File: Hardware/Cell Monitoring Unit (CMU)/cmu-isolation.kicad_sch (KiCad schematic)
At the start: 26 parts, among them T1 CEP99-102, T2 CEP99-102, U1 PESD5V0L2BT, U2 PESD5V0L2BT

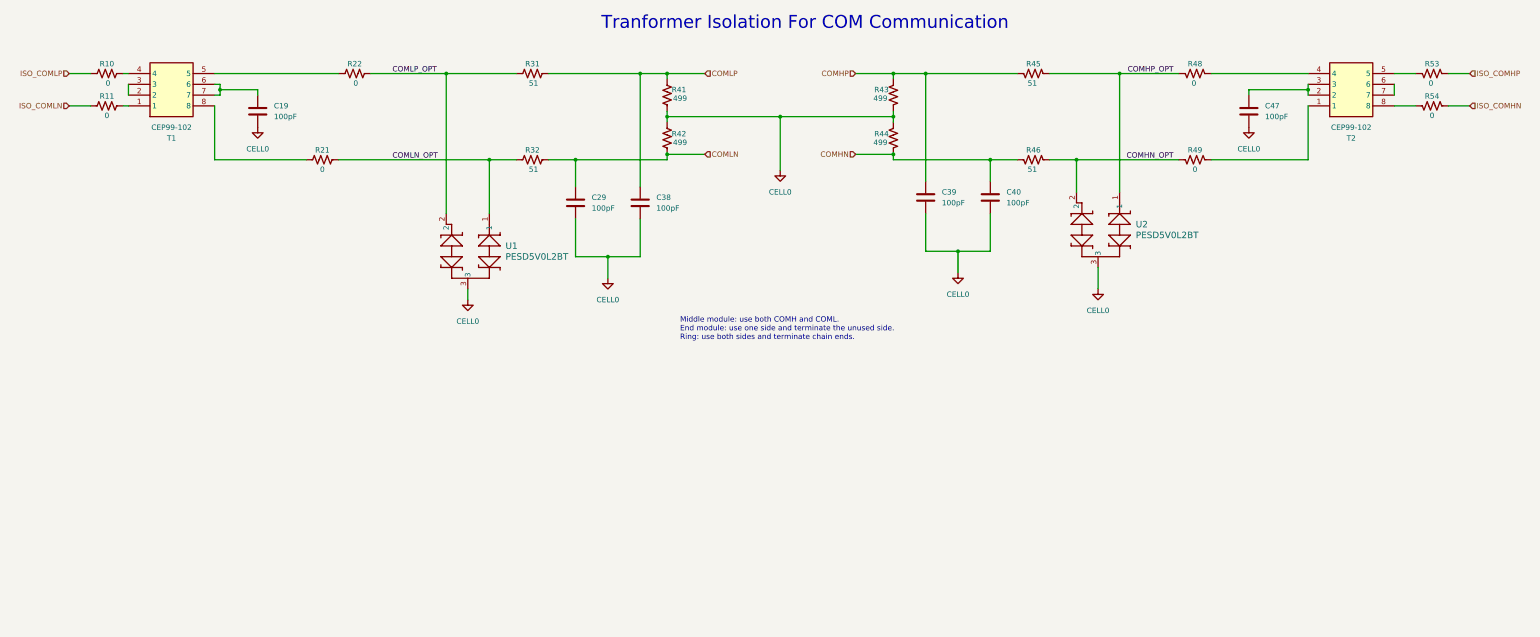
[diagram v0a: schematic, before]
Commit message: updated cmu layout
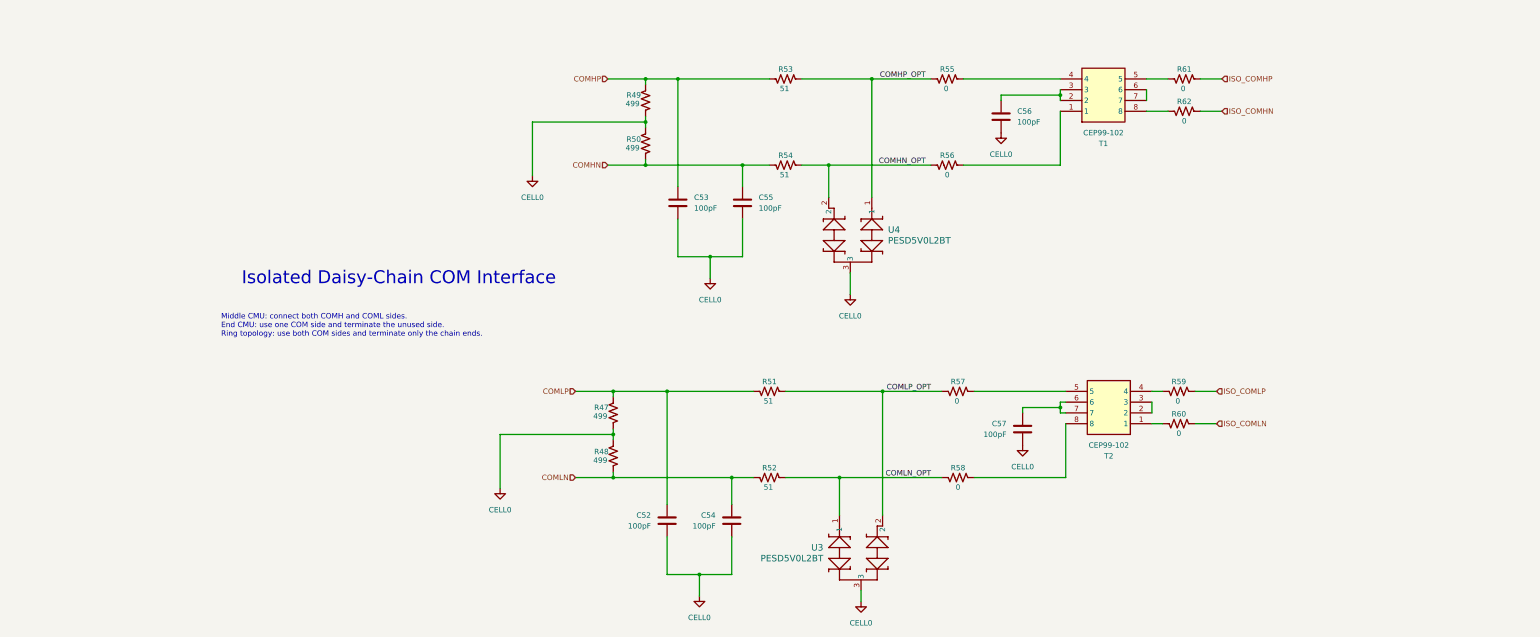
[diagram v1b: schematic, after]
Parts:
- renumbered C38 to C52, C39 to C53, C29 to C54, C40 to C55, C47 to C56, C19 to C57, R41 to R47, R42 to R48, R43 to R49, R44 to R50, R31 to R51, R32 to R52, R45 to R53, R46 to R54, R48 to R55, R49 to R56, R22 to R57, R21 to R58, R10 to R59, R11 to R60, R53 to R61, R54 to R62, T2 to T1, T1 to T2, U1 to U3, U2 to U4
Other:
- note added: "Isolated Daisy-Chain COM Interface"
- note added: "Middle CMU: connect both COMH and COML sides. End CMU: use one COM side and terminate the unused side. Ring topology: use both COM sides and terminate only the chain ends."
- note removed: "Middle module: use both COMH and COML. End module: use one side and terminate the unused side. Ring: use both sides and terminate chain ends."
- note removed: "Tranformer Isolation For COM Communication"
- moved on the sheet: C52, C53, C54, C55, C56, C57, R47, R48, R49, R50, R51, R52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
